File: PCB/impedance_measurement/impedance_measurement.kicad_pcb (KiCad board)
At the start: 2 copper layers, 24 x 25 mm, 26 parts, among them J1 RF_SMD, J2 RF_SMD, J3 20021321-00014C1LF, J4 20021321-00010C4LF, U1 AD8606ARZ, U2 AD5933YRSZ-REEL7, U3 ADP150AUJZ-3.0-R7

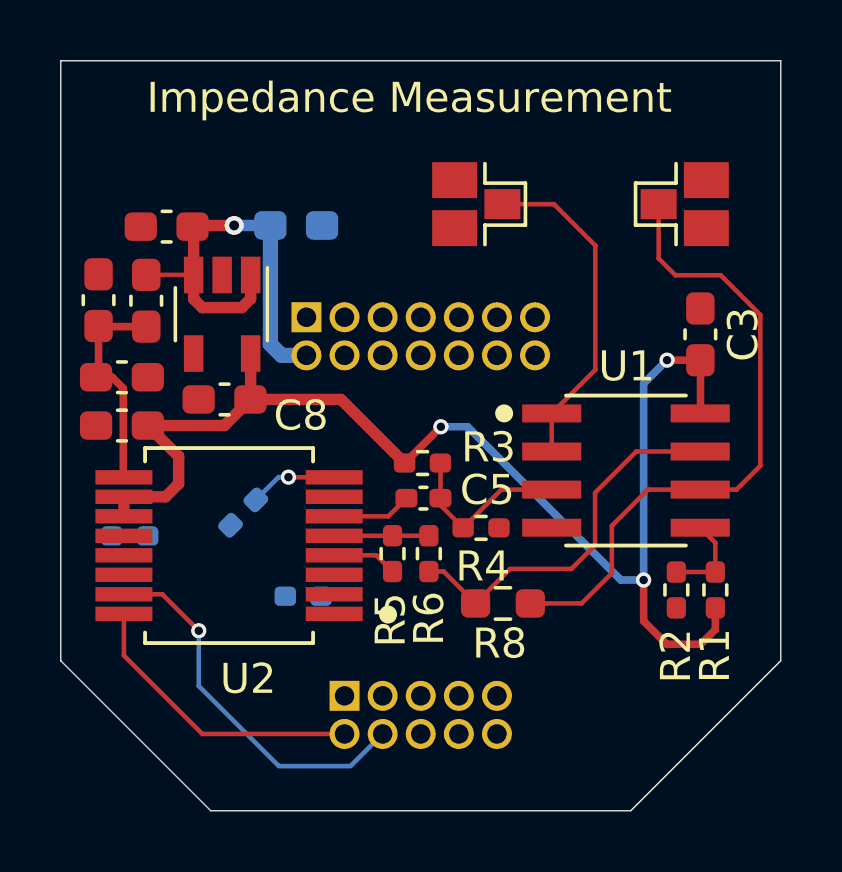
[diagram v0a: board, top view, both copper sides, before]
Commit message: udated by FZ
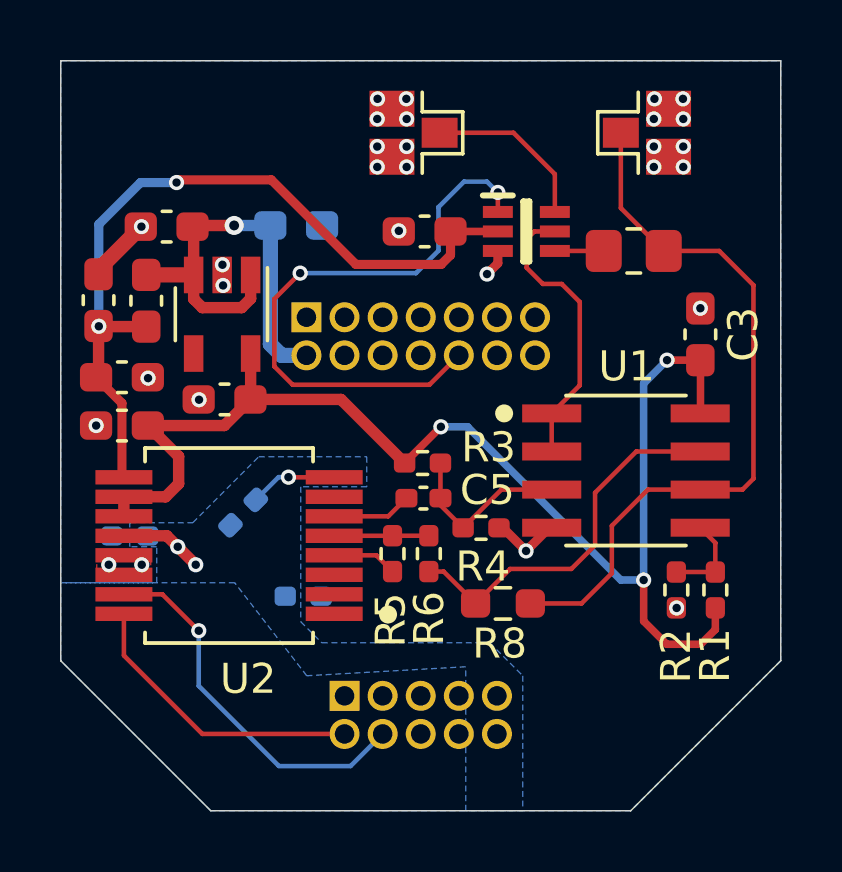
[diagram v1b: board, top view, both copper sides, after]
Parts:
- added C9: 0.1uF, Capacitor_SMD:C_0603_1608Metric_Pad1.08x0.95mm_HandSolder, F.Cu at (132.1, 105.7)
- added R11: 100, Resistor_SMD:R_0805_2012Metric_Pad1.20x1.40mm_HandSolder, F.Cu at (139.1, 106.3)
- added S1: ADG849YKSZ-REEL7, SamacSys_Parts:SOT65P210X110-6N, F.Cu at (135.5, 105.7)
- U2: footprint Mylib:SOP65P780X200-16N -> SOP65P780X200-16N
- moved J1 3.17 mm to (129.4, 102.4)
- moved J2 2.69 mm to (141.9, 102.4)
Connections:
- J1 pad 1: /SIG_OUT -> /SIG_OUT_probe
- J3 pad 10: (no net) -> /Cali_switch
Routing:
- net /Cali_switch: track 0.00 -> 19.8 mm, vias 0 -> 2
- net VDD: track 7.37 -> 26.5 mm, vias 0 -> 2
- net /SIG_OUT_probe: track 0.00 -> 5.67 mm
- net GND: track 0.00 -> 5.50 mm, vias 0 -> 29
- net /SIG_IN: track 21.5 -> 24.5 mm
- net GNDREF: track 0.00 -> 2.79 mm, vias 0 -> 2
- net Net-(R11-Pad1): track 0.00 -> 1.63 mm
- net /SIG_OUT: track 11.1 -> 9.61 mm
- added copper zone on B.Cu, net GND
- added copper zone on F.Cu, net GND
- added copper zone on B.Cu, net GNDREF
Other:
- board text removed: "Impedance Measurement"

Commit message: udated by FZ
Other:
- net class Default removed
